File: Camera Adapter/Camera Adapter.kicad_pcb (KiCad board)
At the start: 2 copper layers, 30 x 50 mm, 13 parts, among them J1 68611514122, J2 634108150321, J3 Conn_01x02, J4 Conn_01x03, J5 68611514122, J6 634108150321, U1 MC33269D-3.3G

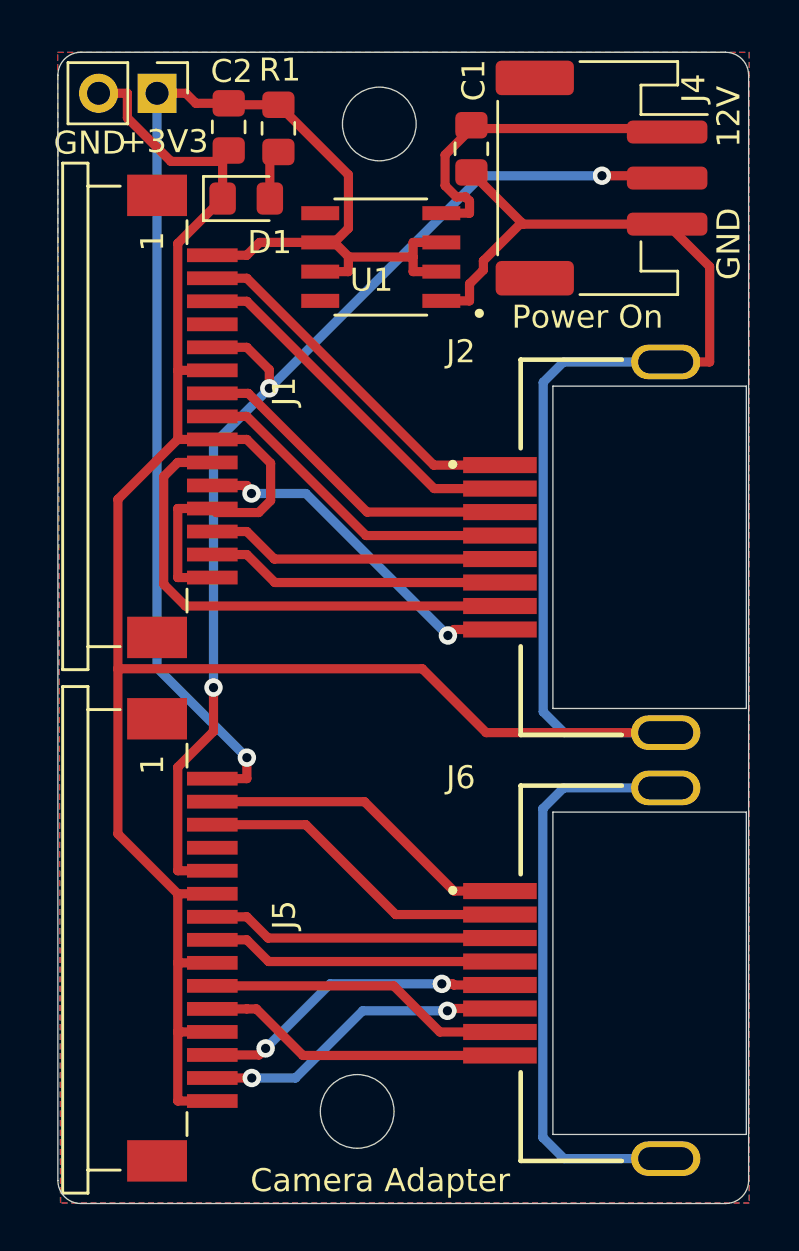
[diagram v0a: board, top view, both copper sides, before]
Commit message: Updated KiCad files
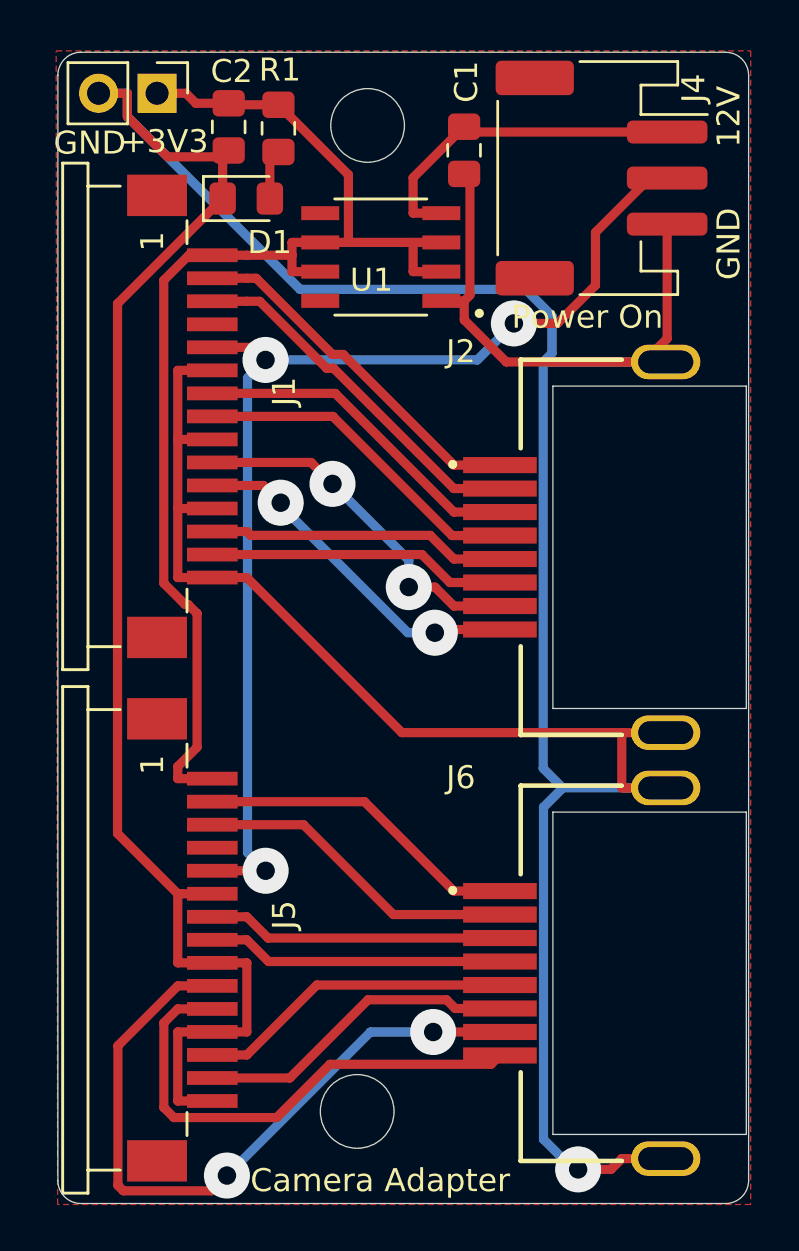
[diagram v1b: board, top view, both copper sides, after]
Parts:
- moved REF2 0.51 mm to (60.5, 31.2)
- moved C1 0.32 mm to (64.6, 32.3)
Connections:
- J6 pad SHIELD1: Net-(J6-PadSHIELD1) -> GND
- J6 pad SHIELD2: Net-(J6-PadSHIELD1) -> GND
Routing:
- net GND: track 148.3 -> 202.5 mm, vias 0 -> 1
- net Net-(J6-PadSHIELD1): track 25.7 -> 0.00 mm
- net CAMERA1DP1: track 13.3 -> 30.8 mm, vias 0 -> 2
- net CAMERA1DN1: track 13.3 -> 21.9 mm
- net +3V3: track 60.7 -> 54.4 mm, vias 1 -> 0
- net CAMERA0DP1: track 22.0 -> 15.8 mm, vias 0 -> 2
- net CAMERAGPIO: track 48.9 -> 49.8 mm
- net CAMERA1DN0: track 13.7 -> 14.1 mm, vias 2 -> 0
- net CAMERA1DP0: vias 2 -> 0
- removed copper zone on B.Cu, net GND
